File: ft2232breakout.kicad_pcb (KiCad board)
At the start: 2 copper layers, 43.2 x 30.5 mm, 34 parts, among them J1 USB_B_Micro, J2 Conn_01x20, J3 Conn_01x20, U1 FT2232H, U2 NCP1117ST33T3G, U3 93LCxxAxxOT, Y1 12MHz

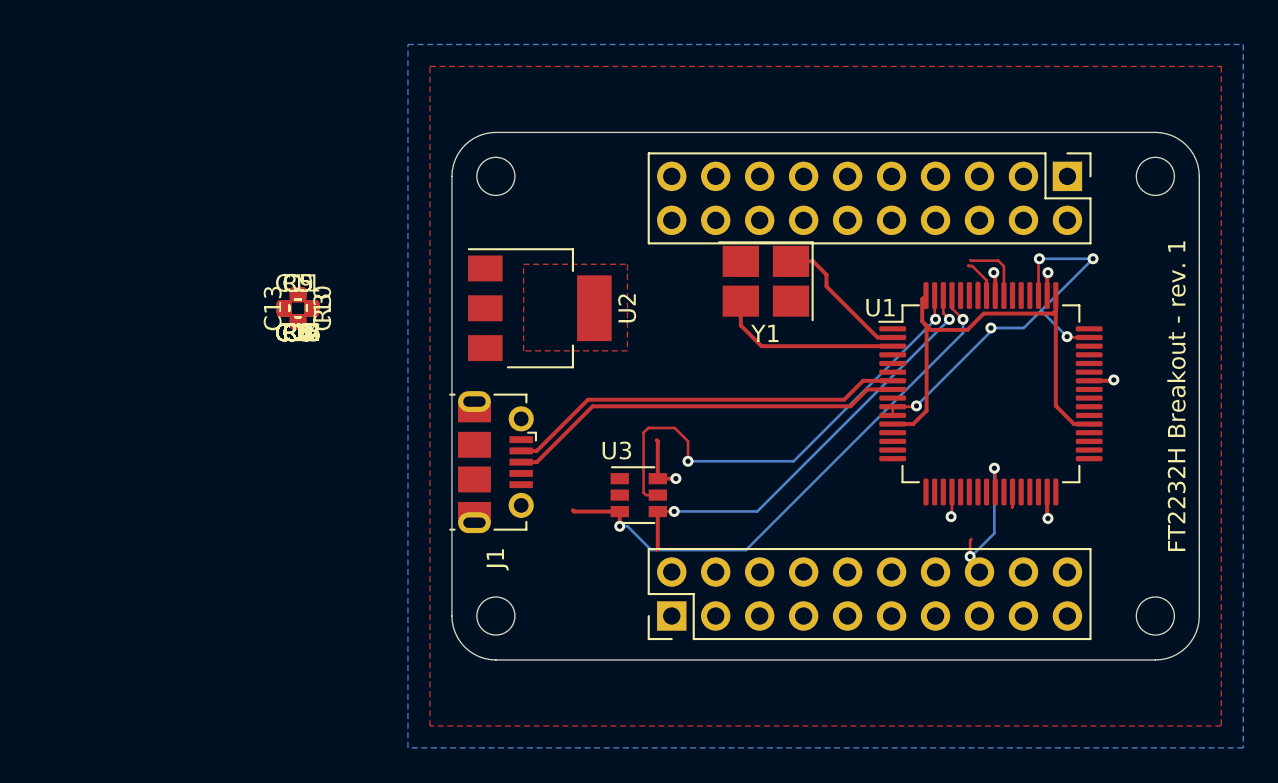
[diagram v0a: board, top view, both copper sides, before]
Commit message: Hmmm
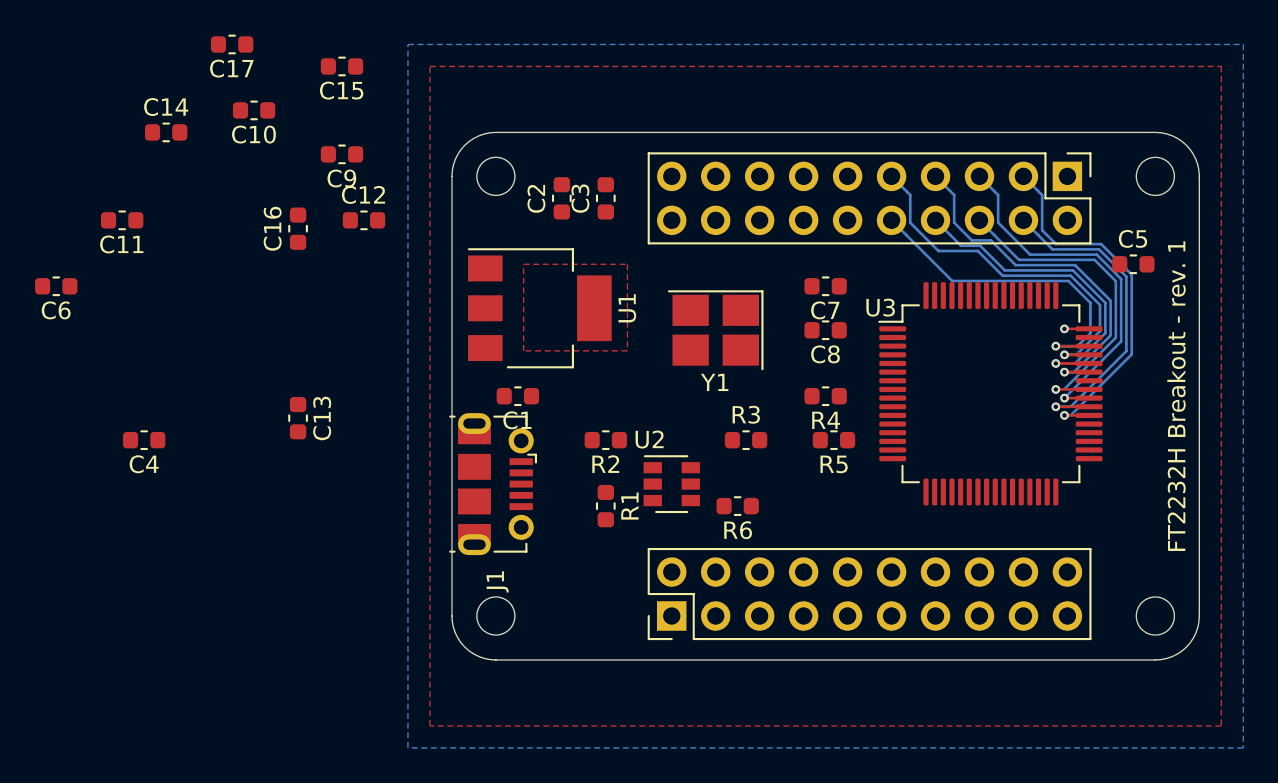
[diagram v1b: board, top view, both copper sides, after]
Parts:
- removed the R5 at (141.0, 99.1)
- added R3: 10k, Resistor_SMD:R_0603_1608Metric, F.Cu at (166.9, 106.7)
- moved C5 48.3 mm to (189.2, 96.5)
- moved R5 31.9 mm to (171.9, 106.7)
- moved R4 30.9 mm to (171.4, 104.1)
- moved C7 30.5 mm to (171.4, 97.8)
- moved C8 30.5 mm to (171.4, 100.3)
- moved R6 27.9 mm to (166.4, 110.5)
- moved R1 21.1 mm to (158.8, 110.5)
- moved R2 19.3 mm to (158.8, 106.7)
- moved C3 18.9 mm to (158.8, 92.7), turned to 90 degrees
- moved C2 16.5 mm to (156.2, 92.7), turned to 90 degrees
- moved C17 15.7 mm to (137.2, 83.8)
- moved C15 14.2 mm to (143.5, 85.1)
- moved C6 14.0 mm to (127.0, 97.8)
- moved C1 13.7 mm to (153.7, 104.1)
- moved C14 12.7 mm to (133.3, 88.9)
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- renumbered C7 to C10, C8 to C11, C9 to C12, C10 to C13, C11 to C14, C12 to C15, C13 to C16, C14 to C17, C17 to C3, C15 to C4, C16 to C6, C3 to C7, C4 to C8, C6 to C9, R3 to R1, R4 to R2, R1 to R4, R2 to R5, U2 to U1, U3 to U2, U1 to U3
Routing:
- net GND: track 32.6 -> 0.00 mm, vias 7 -> 0
- net Net-(R1-Pad2): track 31.6 -> 0.00 mm, vias 2 -> 0
- net Net-(R6-Pad1): track 27.6 -> 0.00 mm, vias 2 -> 0
- net +1V8: track 26.9 -> 0.00 mm
- net Net-(R3-Pad1): track 25.2 -> 0.00 mm, vias 2 -> 0
- net Net-(J1-Pad3): track 23.2 -> 0.00 mm
- net Net-(J1-Pad2): track 23.1 -> 0.00 mm
- net /BD6: track 0.00 -> 21.6 mm, vias 0 -> 1
- net /BD2: track 0.00 -> 21.2 mm, vias 0 -> 1
- net /BD0: track 0.00 -> 21.2 mm, vias 0 -> 1
- net /BD4: track 0.00 -> 21.0 mm, vias 0 -> 1
- net /BD7: track 0.00 -> 19.5 mm, vias 0 -> 1
- net /BD3: track 0.00 -> 19.2 mm, vias 0 -> 1
- net /BD5: track 0.00 -> 19.0 mm, vias 0 -> 1
- net /BD1: track 0.00 -> 18.9 mm, vias 0 -> 1
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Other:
- net class Default: via_dia 0.635 -> 0.508; via_drill 0.3 -> 0.254
- rule via_min_drill: 0.3 -> 0.254
- rule via_min_size: 0.4 -> 0.508
